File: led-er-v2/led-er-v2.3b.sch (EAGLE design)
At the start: 39 parts, among them IC1 TLC59711, IC2 TLC59711, IC3 TLC59711, IC4 TLC59711

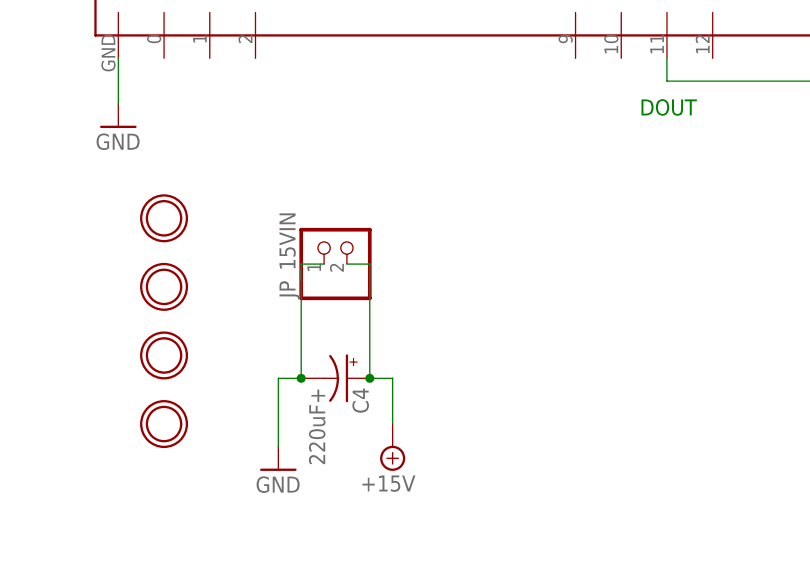
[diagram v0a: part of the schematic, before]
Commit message: updated led-er 2.3b
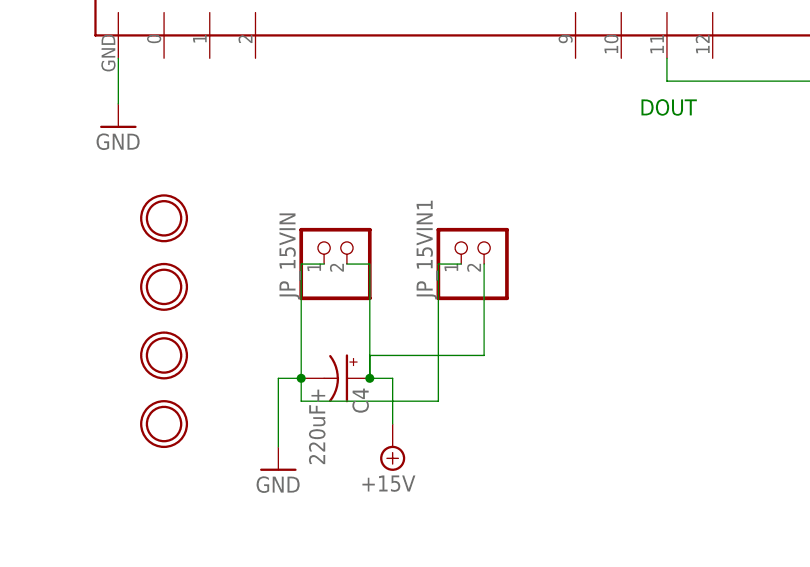
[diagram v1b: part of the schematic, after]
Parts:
- added JP_15VIN1: (no value), microbuilder:HEADER-1X2
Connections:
- net +15V: now also JP_15VIN1.2
- net GND: now also JP_15VIN1.1
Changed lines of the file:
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@@
 <?xml version="1.0" encoding="utf-8"?>
 <!DOCTYPE eagle SYSTEM "eagle.dtd">
-<eagle version="7.2.0">
+<eagle version="7.5.0">
 <drawing>
 <settings>
@@
 <part name="JP_SIGIN" library="microbuilder" deviceset="HEADER-1X2" device=""/>
 <part name="U$6" library="Andrews" deviceset="HEADER-2X8-RIBBON" device=""/>
+<part name="JP_15VIN1" library="microbuilder" deviceset="HEADER-1X2" device=""/>
 </parts>
 <sheets>
@@
 <instance part="JP_SIGIN" gate="G$1" x="60.96" y="40.64" rot="R90"/>
 <instance part="U$6" gate="G$1" x="104.14" y="-58.42" rot="R90"/>
+<instance part="JP_15VIN1" gate="G$1" x="-7.62" y="-35.56" rot="R90"/>
 </instances>
 <busses>
@@
 <wire x1="-30.48" y1="-50.8" x2="-30.48" y2="-58.42" width="0.1524" layer="91"/>
 <junction x="-27.94" y="-50.8"/>
+<pinref part="JP_15VIN1" gate="G$1" pin="1"/>
+<wire x1="-10.16" y1="-38.1" x2="-12.7" y2="-38.1" width="0.1524" layer="91"/>
+<wire x1="-12.7" y1="-38.1" x2="-12.7" y2="-53.34" width="0.1524" layer="91"/>
+<wire x1="-12.7" y1="-53.34" x2="-27.94" y2="-53.34" width="0.1524" layer="91"/>
+<wire x1="-27.94" y1="-53.34" x2="-27.94" y2="-50.8" width="0.1524" layer="91"/>
 </segment>
 </net>
@@
 <wire x1="-17.78" y1="-50.8" x2="-17.78" y2="-55.88" width="0.1524" layer="91"/>
 <junction x="-20.32" y="-50.8"/>
-</segment>
-<segment>
+<pinref part="JP_15VIN1" gate="G$1" pin="2"/>
+<wire x1="-7.62" y1="-38.1" x2="-7.62" y2="-48.26" width="0.1524" layer="91"/>
+<wire x1="-7.62" y1="-48.26" x2="-20.32" y2="-48.26" width="0.1524" layer="91"/>
+<wire x1="-20.32" y1="-48.26" x2="-20.32" y2="-50.8" width="0.1524" layer="91"/>
+</segment>
+<segment>
